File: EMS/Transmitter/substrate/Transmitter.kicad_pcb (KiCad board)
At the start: 2 copper layers, 60 x 60 mm, 12 parts

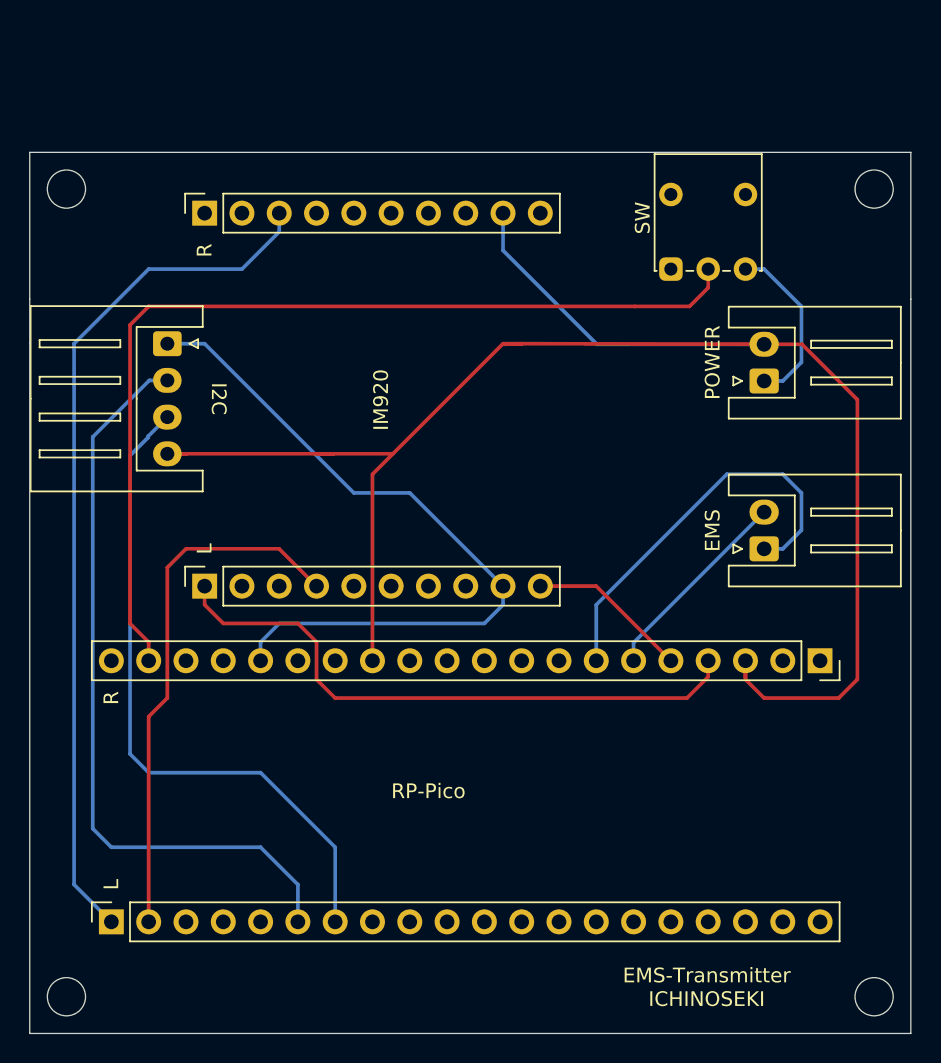
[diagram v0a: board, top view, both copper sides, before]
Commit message: Update transmitter.
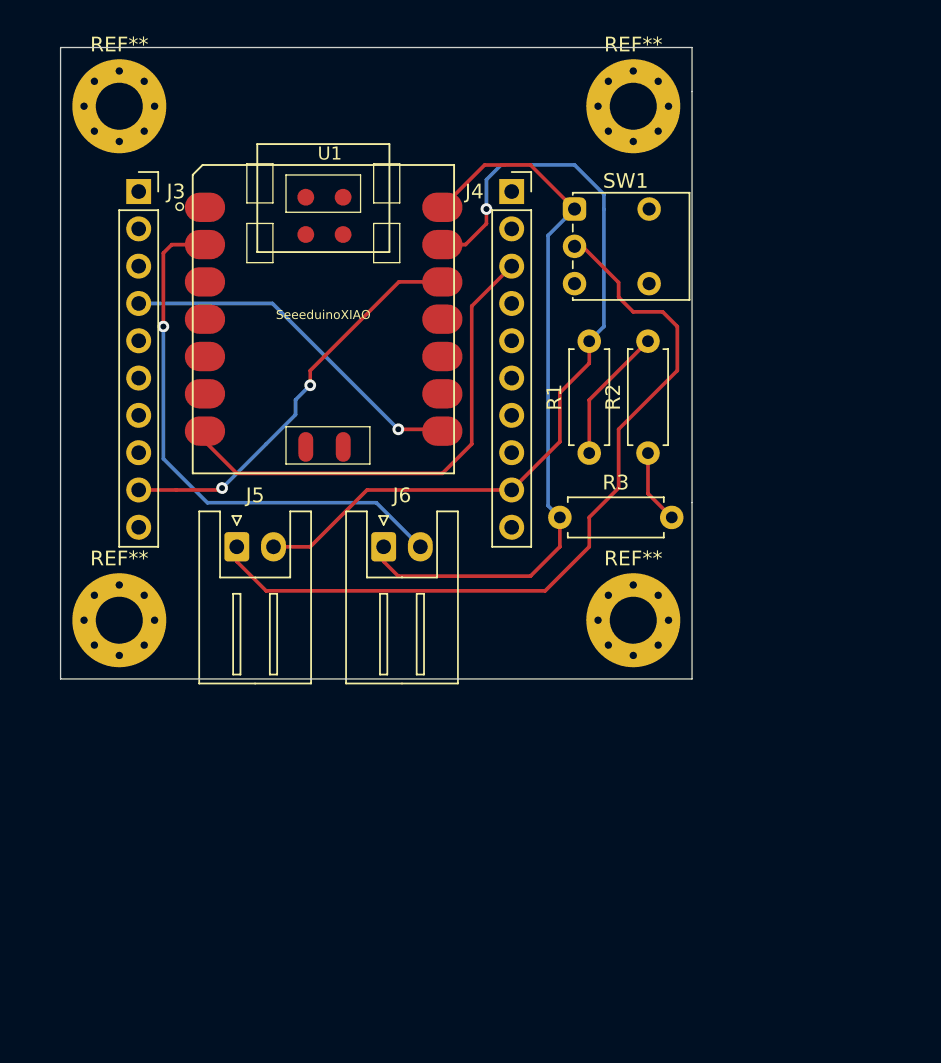
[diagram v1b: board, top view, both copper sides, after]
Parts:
- removed I2C: I2C, Connector_JST:JST_XH_S4B-XH-A_1x04_P2.50mm_Horizontal
- removed L: Pico_Left, Connector_PinSocket_2.54mm:PinSocket_1x20_P2.54mm_Vertical
- removed R: Pico_Right, Connector_PinSocket_2.54mm:PinSocket_1x20_P2.54mm_Vertical
- removed the REF** at (176.4, 134.6)
- removed the REF** at (176.4, 79.6)
- removed the REF** at (121.4, 79.6)
- removed the REF** at (121.4, 134.6)
- added R1: 18Ω, Resistor_THT:R_Axial_DIN0207_L6.3mm_D2.5mm_P7.62mm_Horizontal, F.Cu at (157.0, 97.6)
- added R2: 18Ω, Resistor_THT:R_Axial_DIN0207_L6.3mm_D2.5mm_P7.62mm_Horizontal, F.Cu at (161.0, 97.6)
- added R3: 18Ω, Resistor_THT:R_Axial_DIN0207_L6.3mm_D2.5mm_P7.62mm_Horizontal, F.Cu at (155.0, 102.0)
- added REF**: MountingHole_3.2mm_M3_Pad_Via, MountingHole:MountingHole_3.2mm_M3_Pad_Via, F.Cu at (160.0, 109.0)
- added REF**: MountingHole_3.2mm_M3_Pad_Via, MountingHole:MountingHole_3.2mm_M3_Pad_Via, F.Cu at (125.0, 109.0)
- added REF**: MountingHole_3.2mm_M3_Pad_Via, MountingHole:MountingHole_3.2mm_M3_Pad_Via, F.Cu at (160.0, 74.0)
- added REF**: MountingHole_3.2mm_M3_Pad_Via, MountingHole:MountingHole_3.2mm_M3_Pad_Via, F.Cu at (125.0, 74.0)
- added U1: SeeeduinoXIAO, Seeeduino XIAO KICAD:Seeeduino XIAO-MOUDLE14P-2.54-21X17.8MM, F.Cu at (130.0, 99.0)
- J3: renamed from L; value ADP_Left -> ADP_L
- J4: renamed from R; value ADP_Right -> ADP_R
- J6: renamed from EMS; value EMS_IN -> ESS_IN
- moved J5 37.6 mm to (133.0, 104.0), turned to 0 degrees
- moved J3 27.2 mm to (126.3, 79.8), turned to 0 degrees
- moved J6 25.9 mm to (143.0, 104.0), turned to 0 degrees
- moved J4 21.0 mm to (151.7, 79.8), turned to 0 degrees
- moved SW1 7.73 mm to (156.0, 81.0), turned to 0 degrees
- renumbered POWER to J5, SW to SW1
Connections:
- J3 pad 1: Net-(J2-Pad4) -> (no net)
- J3 pad 10: Net-(J2-Pad5) -> (no net)
- J3 pad 2: Net-(J3-Pad2) -> (no net)
- J3 pad 3: Net-(J3-Pad3) -> (no net)
- J3 pad 4: Net-(J1-Pad2) -> RX
- J3 pad 5: Net-(J3-Pad5) -> (no net)
- J3 pad 6: Net-(J3-Pad6) -> (no net)
- J3 pad 7: Net-(J3-Pad7) -> (no net)
- J3 pad 8: Net-(J3-Pad8) -> (no net)
- J3 pad 9: Net-(J2-Pad16) -> +3V3
- J4 pad 1: Net-(J4-Pad1) -> (no net)
- J4 pad 10: Net-(J4-Pad10) -> (no net)
- J4 pad 2: Net-(J4-Pad2) -> (no net)
- J4 pad 3: Net-(J1-Pad1) -> TX
- J4 pad 4: Net-(J4-Pad4) -> (no net)
- J4 pad 5: Net-(J4-Pad5) -> (no net)
- J4 pad 6: Net-(J4-Pad6) -> (no net)
- J4 pad 7: Net-(J4-Pad7) -> (no net)
- J4 pad 8: Net-(J4-Pad8) -> (no net)
- J5 pad 1: +5V -> PW_IN
- J6 pad 1: Net-(J2-Pad7) -> +5V
- J6 pad 2: Net-(J2-Pad6) -> ESS_IN
- SW1 pad 1: Net-(SW1-Pad1) -> +5V
- SW1 pad 2: Net-(J2-Pad19) -> PW_IN
- SW1 pad 3: +5V -> (no net)
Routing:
- net GND: track 123.0 -> 56.4 mm, vias 0 -> 1
- net Net-(J2-Pad19): track 65.1 -> 0.00 mm
- net Net-(J1-Pad1): track 58.8 -> 0.00 mm
- net PW_IN: track 0.00 -> 54.4 mm
- net Net-(J1-Pad6): track 51.4 -> 0.00 mm
- net Net-(J2-Pad16): track 49.8 -> 0.00 mm
- net Net-(J1-Pad7): track 45.7 -> 0.00 mm
- net Net-(J2-Pad4): track 41.4 -> 0.00 mm
- net +5V: track 11.7 -> 49.8 mm
- net ESS_IN: track 0.00 -> 37.1 mm, vias 0 -> 1
- net Net-(J1-Pad2): track 36.4 -> 0.00 mm
- net TX: track 0.00 -> 33.8 mm
- net +3V3: track 0.00 -> 27.7 mm, vias 0 -> 2
- net Net-(J2-Pad7): track 27.6 -> 0.00 mm
- net RX: track 0.00 -> 24.3 mm, vias 0 -> 1
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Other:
- board size 60 x 60 mm -> 43 x 43 mm
- board text removed: "EMS-Transmitter ICHINOSEKI"
- board text removed: "IM920"
- board text removed: "RP-Pico"
